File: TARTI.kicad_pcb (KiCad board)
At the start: 2 copper layers, 37.9 x 47.2 mm, 7 parts, among them J1 Conn_01x04_Socket, J2 Conn_01x04_Socket, J3 Screw_Terminal_01x02, U1 LM7805_TO220

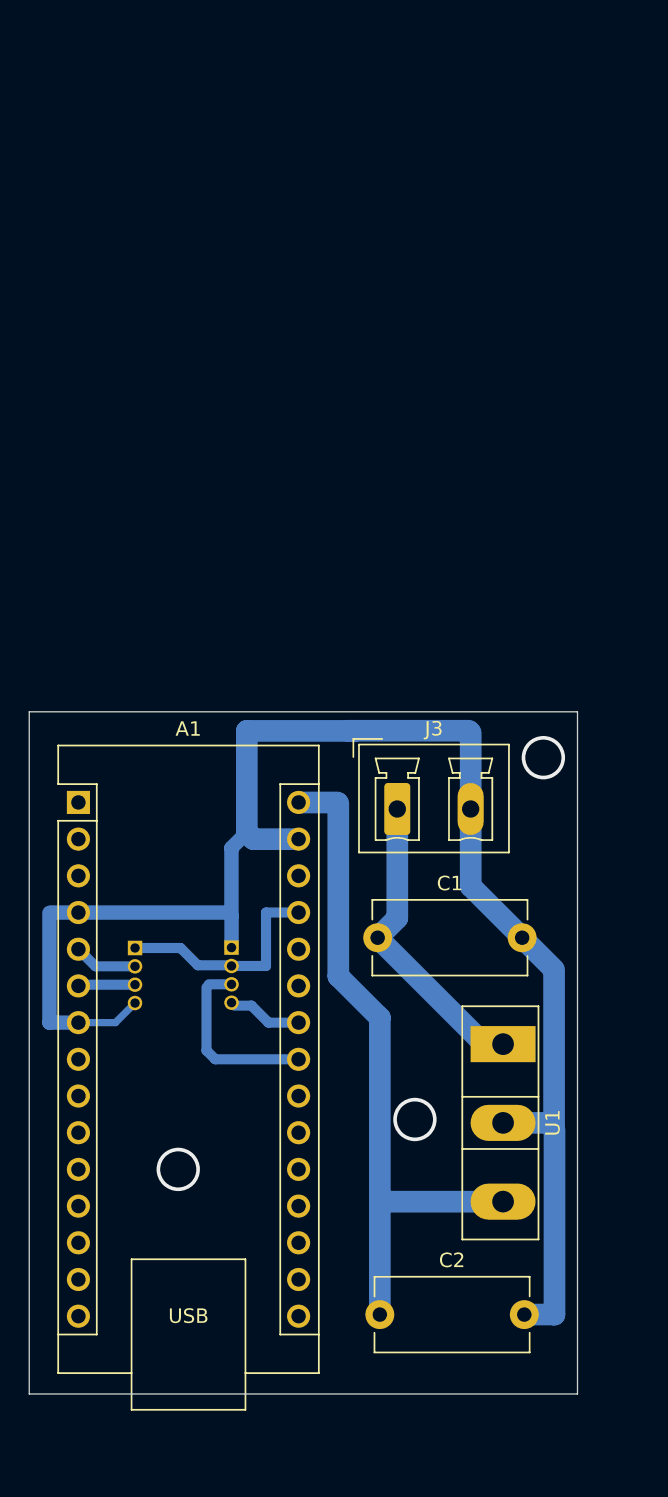
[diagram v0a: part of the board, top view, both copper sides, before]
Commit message: Add files via upload
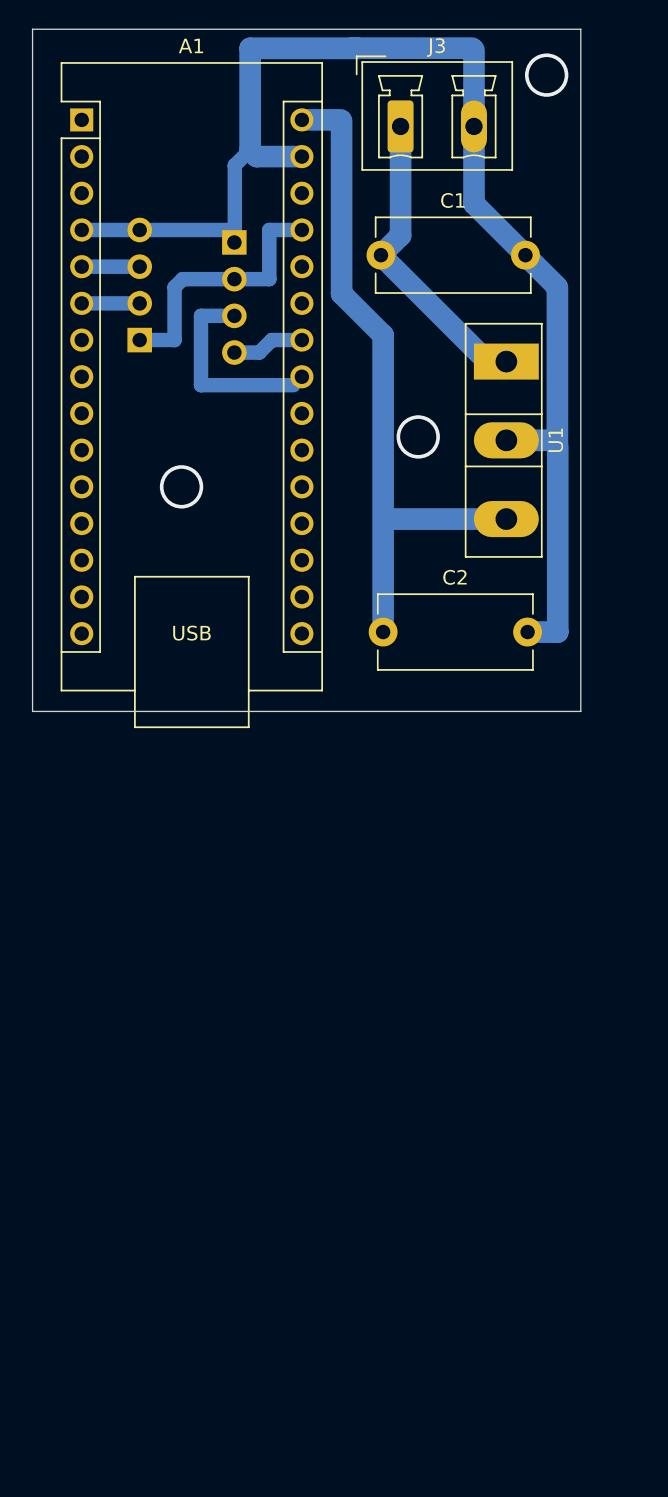
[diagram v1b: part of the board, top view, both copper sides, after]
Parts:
- J1, J2: footprint Connector_PinHeader_1.27mm:PinHeader_1x04_P1.27mm_Vertical -> Connector_PinSocket_2.54mm:PinSocket_1x04_P2.54mm_Vertical
- moved J2 48.8 mm to (14.2, -32.5)
- moved A1 47.2 mm to (3.61, -40.9)
- moved C1 47.2 mm to (24.3, -31.6)
- moved C2 47.2 mm to (24.5, -5.50)
- moved J3 47.2 mm to (25.7, -40.5)
- moved U1 47.2 mm to (33.0, -24.2)
- moved J1 42.1 mm to (7.62, -25.7), turned to 0 degrees
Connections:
- A1 pad 7: GND -> unconnected-(A1-D4-Pad7)
- J1 pad 2: D3 -> D2
- J1 pad 3: D2 -> D3
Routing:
- net GND: track 116.5 -> 98.8 mm
- net 5V: track 15.5 -> 18.9 mm
- net A4: track 12.9 -> 14.3 mm
- net D2: track 3.95 -> 4.49 mm
